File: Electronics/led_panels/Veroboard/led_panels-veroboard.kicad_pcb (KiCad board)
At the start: 2 copper layers, 91.4 x 160 mm, 113 parts, among them P1 CONN_2

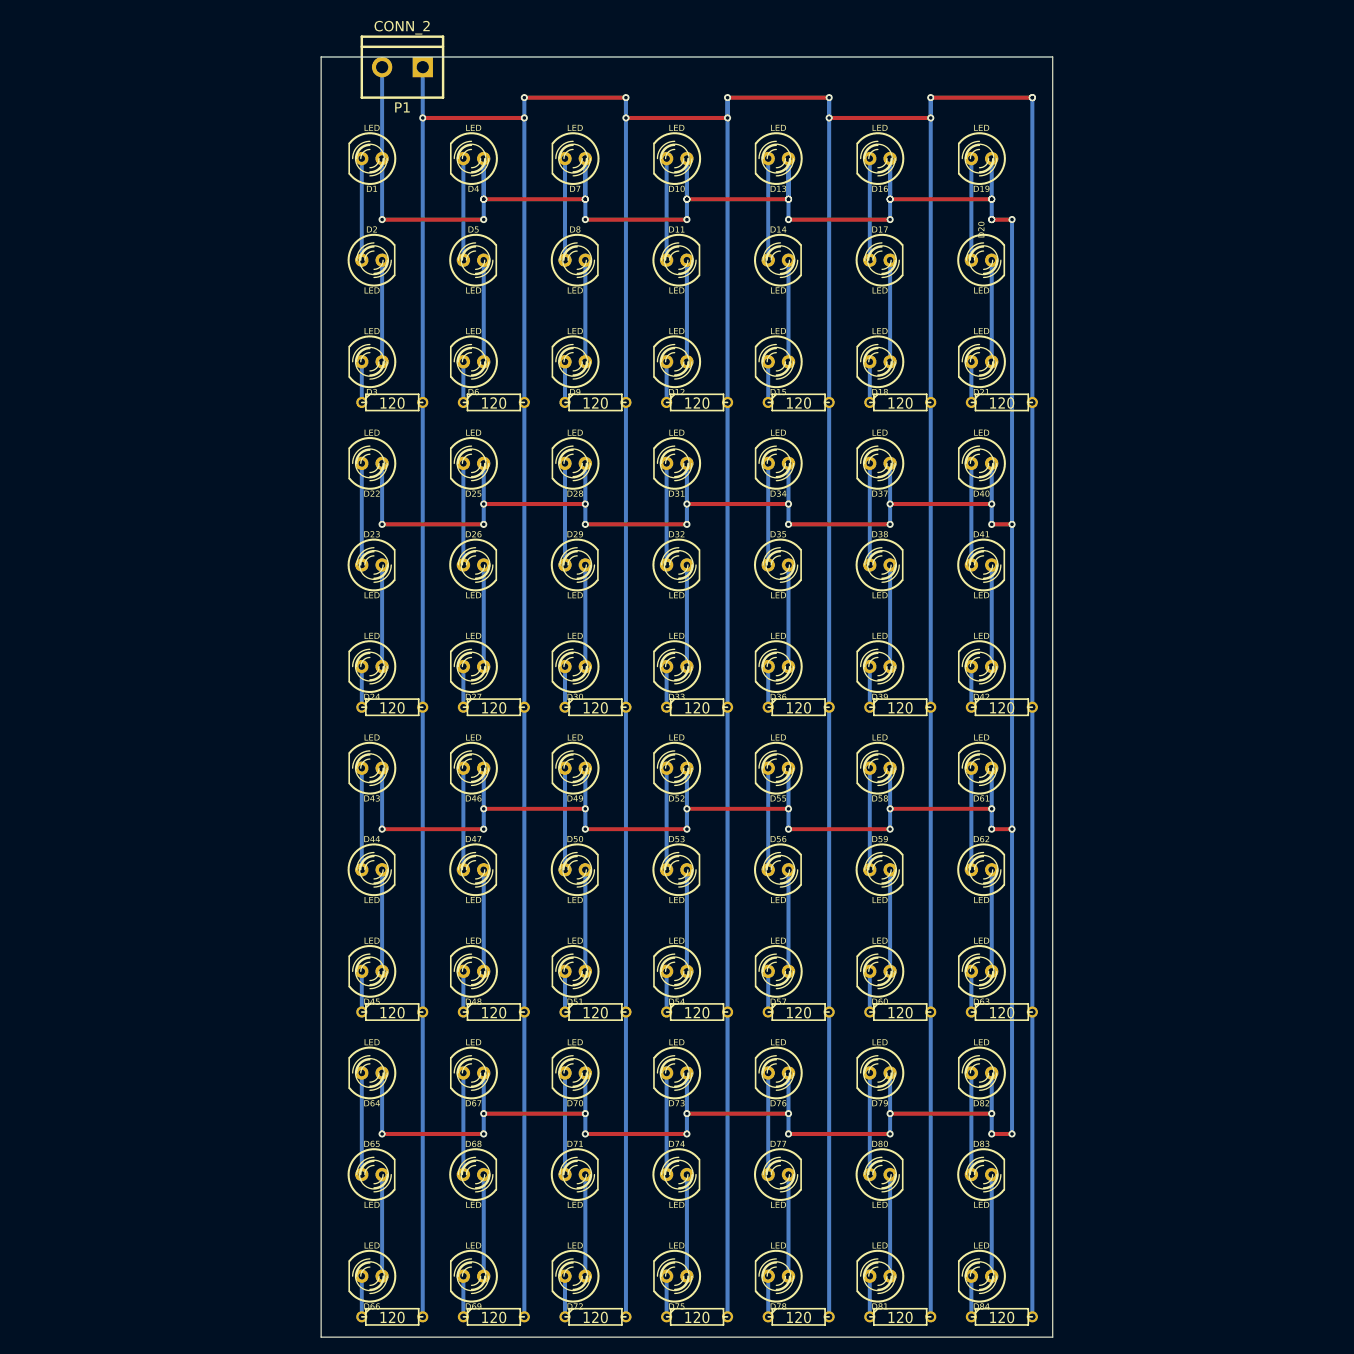
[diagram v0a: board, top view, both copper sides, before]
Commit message: Changes for v1.1
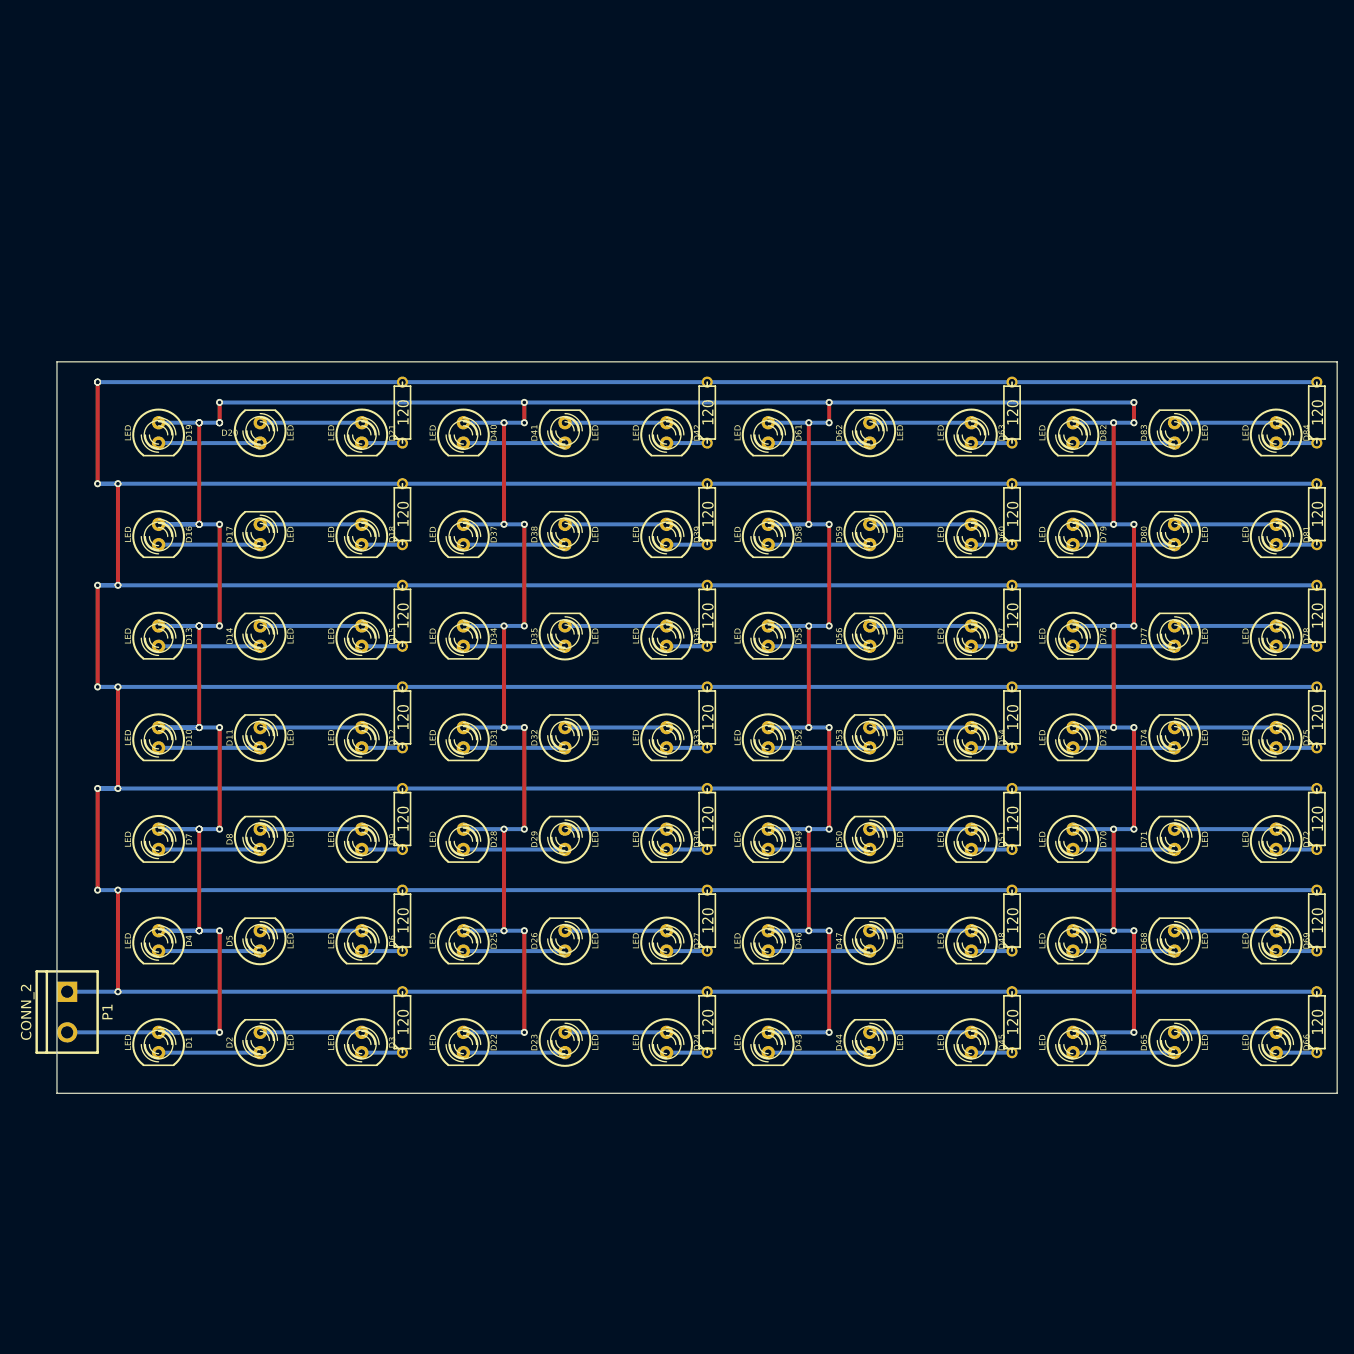
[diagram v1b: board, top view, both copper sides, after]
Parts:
- moved P1 125.3 mm to (26.7, 177.8), turned to 270 degrees
- moved R22 121.3 mm to (182.9, 179.1), turned to 90 degrees
- moved R28 119.7 mm to (182.9, 102.9), turned to 90 degrees
- moved D66 116.7 mm to (177.8, 181.6), turned to 270 degrees
- moved R23 114.2 mm to (182.9, 166.4), turned to 90 degrees
- moved D1 113.7 mm to (38.1, 181.6), turned to 270 degrees
- moved R27 113.0 mm to (182.9, 115.6), turned to 90 degrees
- moved D84 111.7 mm to (177.8, 105.4), turned to 270 degrees
- moved R24 109.6 mm to (182.9, 153.7), turned to 90 degrees
- moved R26 109.0 mm to (182.9, 128.3), turned to 90 degrees
- moved D69 108.7 mm to (177.8, 168.9), turned to 270 degrees
- moved D19 108.4 mm to (38.1, 105.4), turned to 270 degrees
- moved R25 107.8 mm to (182.9, 141.0), turned to 90 degrees
- moved D4 105.4 mm to (38.1, 168.9), turned to 270 degrees
- moved D81 105.1 mm to (177.8, 118.1), turned to 270 degrees
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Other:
- board size 91.4 x 160 mm -> 160 x 91.4 mm
